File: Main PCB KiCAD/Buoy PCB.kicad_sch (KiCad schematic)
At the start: 4 parts, among them J1 Front B, J2 Front A, J3 Back B, J4 Back A

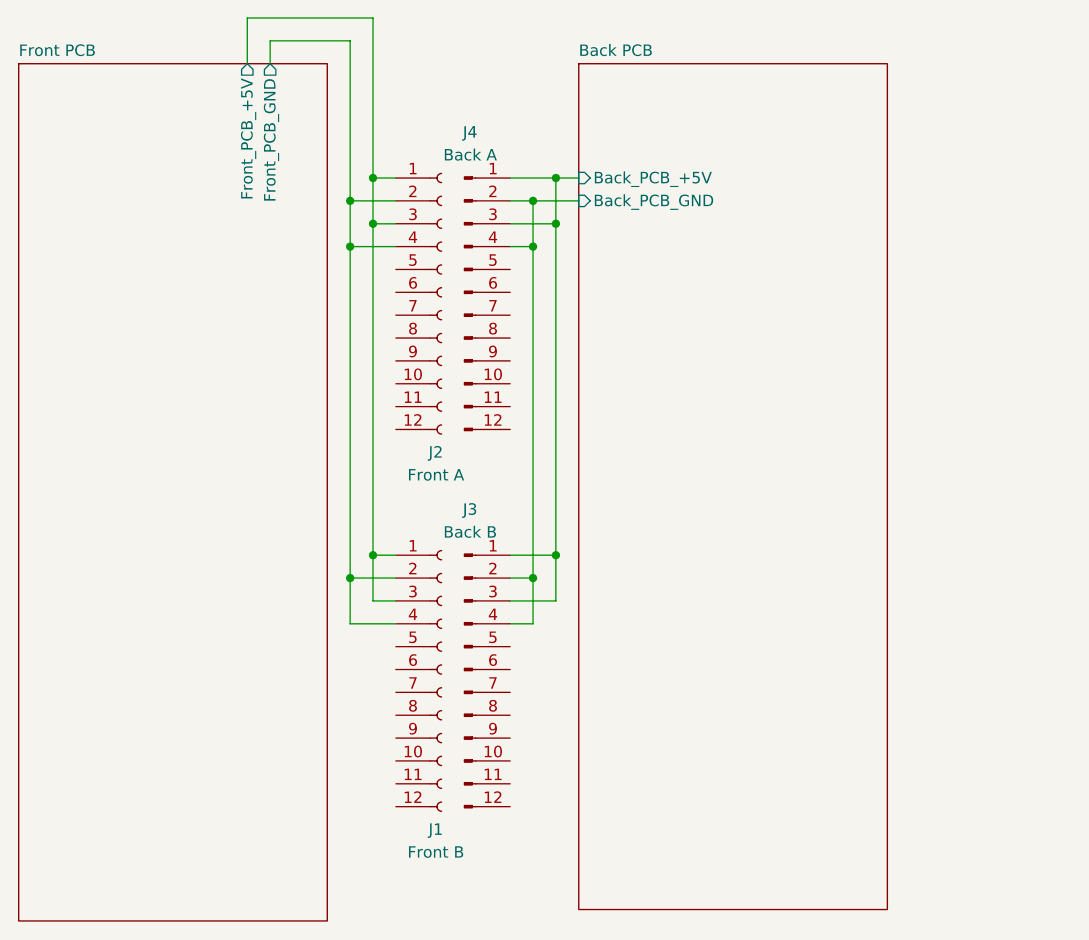
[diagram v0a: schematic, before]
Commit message: .
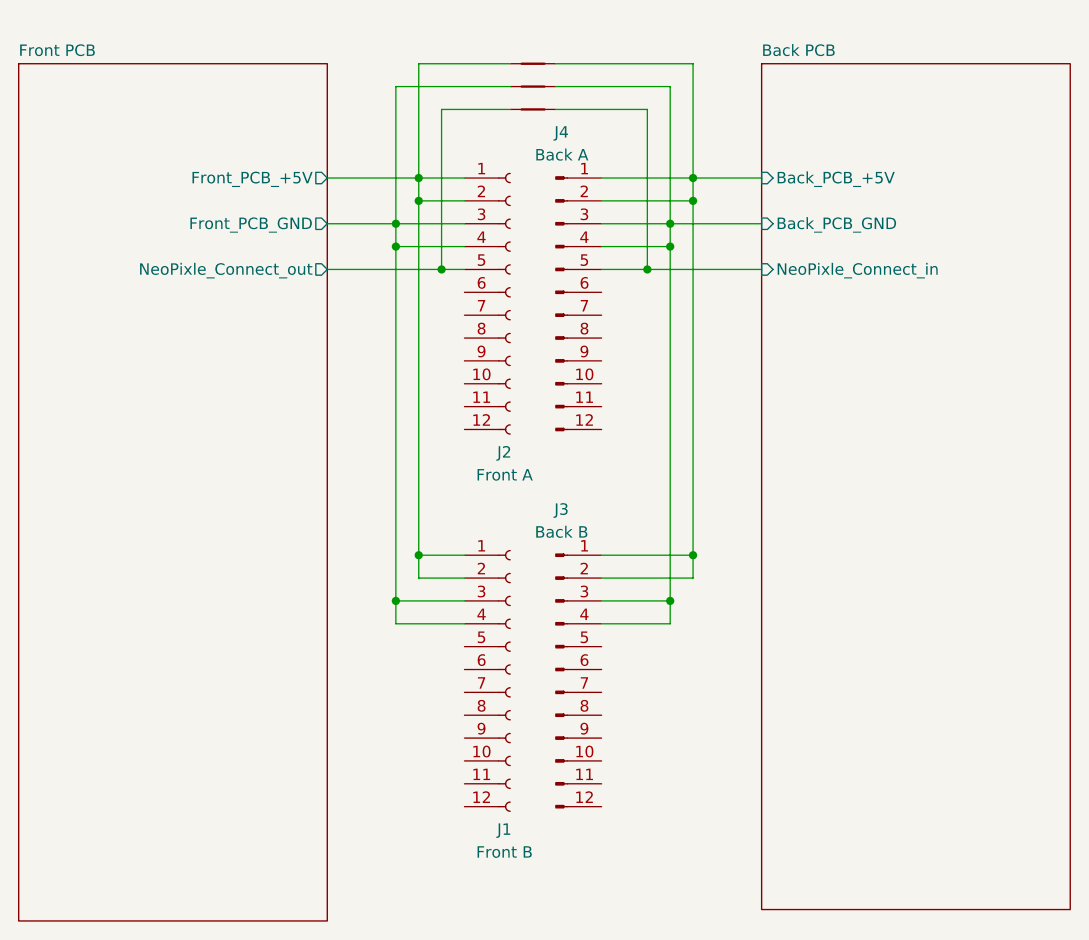
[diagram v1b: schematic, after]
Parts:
- added NT1, NT2, NT3: NetTie_2, NetTie:NetTie-2_SMD_Pad0.5mm, symbol Device:NetTie_2
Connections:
- net Back PCB/Back_PCB_+5V: now also J3.2 (Pin_2), J4.2 (Pin_2), NT2.2; no longer J3.3 (Pin_3), J4.3 (Pin_3)
- net Back PCB/Back_PCB_GND: now also J3.3 (Pin_3), J4.3 (Pin_3), NT1.2; no longer J3.2 (Pin_2), J4.2 (Pin_2)
- net Front PCB/Front_PCB_+5V: now also J1.2 (Pin_2), J2.2 (Pin_2), NT2.1; no longer J1.3 (Pin_3), J2.3 (Pin_3)
- net Front PCB/Front_PCB_GND: now also J1.3 (Pin_3), J2.3 (Pin_3), NT1.1; no longer J1.2 (Pin_2), J2.2 (Pin_2)
- net Back PCB/NeoPixle_Connect_in: now reaches J4.5 (Pin_5)
- net Back PCB/NeoPixle_Connect_in: now also NT3.2
- net Front PCB/NeoPixle_Connect_out: now reaches J2.5 (Pin_5)
- net Front PCB/NeoPixle_Connect_out: now also NT3.1
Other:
- sheet Back PCB ports: added NeoPixle_Connect_in; removed none
- sheet Front PCB ports: added NeoPixle_Connect_out; removed none
- moved on the sheet: J1, J2, J3, J4
